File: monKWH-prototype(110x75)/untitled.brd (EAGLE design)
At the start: 69.4 x 109.6 mm, 26 parts, among them J1 U.FL-R-SMT(01), X1 MSTBA2

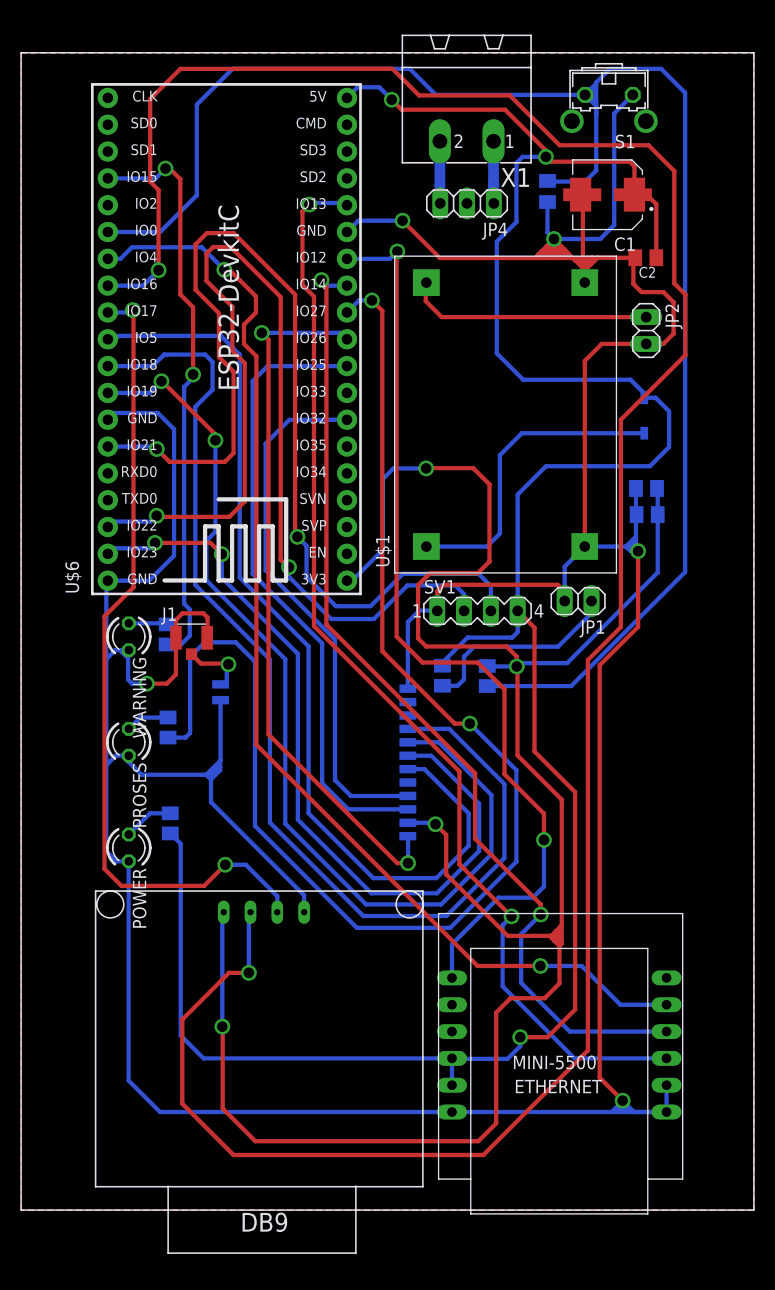
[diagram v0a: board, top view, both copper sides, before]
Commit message: perubahan mikro dan penambahan Jack-DC
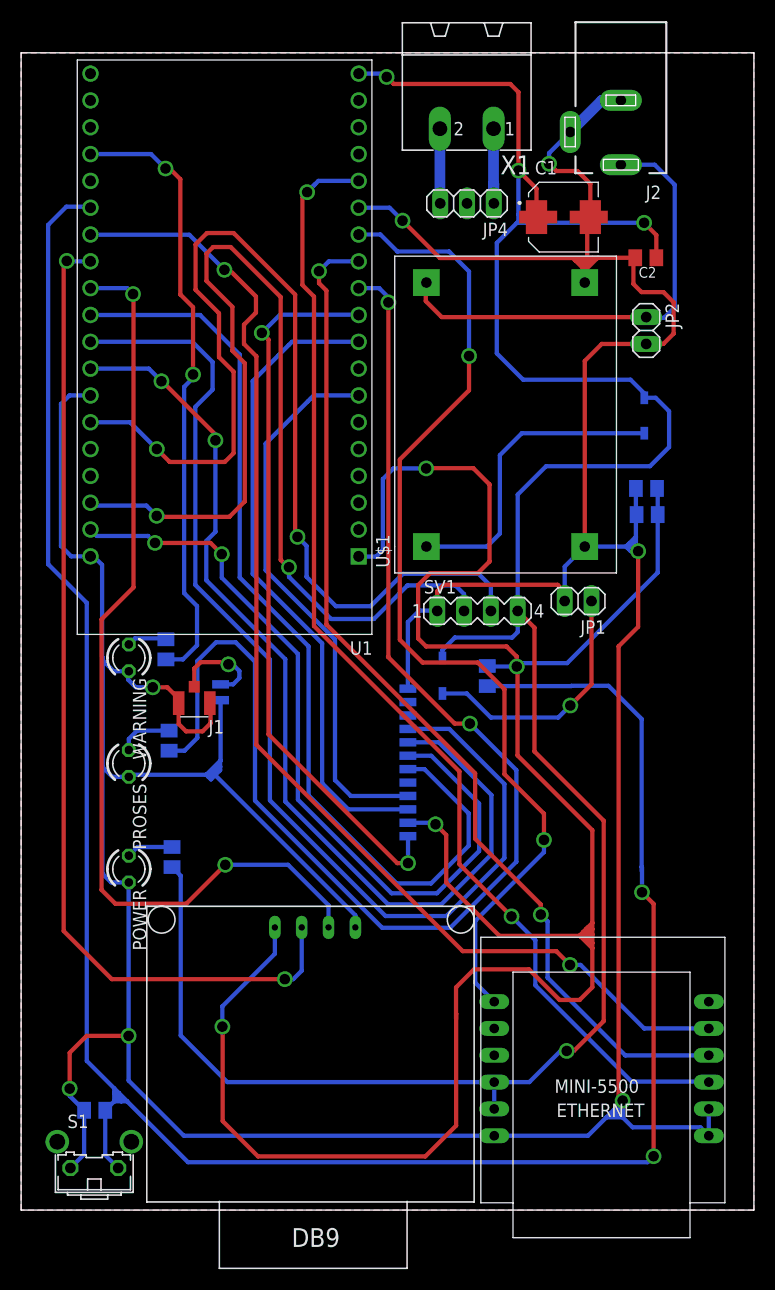
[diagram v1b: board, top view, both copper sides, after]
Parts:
- removed U$6: ESP32DEVKITC, ESP32-DEVKITC:ESP32-DEVKITC
- added J2: DCJ0202, con-jack:DCJ0202
- added U1: ESP32-DEVKITC-32D, ESP32-DEVKITC-32D:MODULE_ESP32-DEVKITC-32D
- R2: device adafruit:M0805 -> 1N5819HW-7:SOD3715X145N
- moved S1 110.5 mm to (3.73, 3.93), turned to 0 degrees
- moved C3 97.0 mm to (3.77, 8.15), turned to 0 degrees
- moved J1 6.19 mm to (13.2, 46.7), turned to 180 degrees
- moved U$5 5.06 mm to (39.7, 27.5)
- moved C1 4.69 mm to (48.2, 92.7), turned to 0 degrees
- moved U$3 4.59 mm to (63.5, -0.61)
- moved R1 3.19 mm to (11.1, 32.1)
- moved POWER 2.00 mm to (7.00, 31.0)
- moved PROSES 2.00 mm to (7.00, 41.0)
- moved WARNING 2.00 mm to (7.00, 51.0)
- moved R16 1.41 mm to (10.5, 51.8)
- moved R3 1.25 mm to (10.8, 43.2)
- moved X1 1.19 mm to (39.0, 106.2)
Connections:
- removed net EN: U$6.2
- removed net RST_LAN1: U$6.8
- net 3V3: now also U1.1; no longer U$6.1
- net GND: now also J2.2, J2.3, U1.14, U1.20, U1.26; no longer U$6.14, U$6.32, U$6.38
- net LED_PROSES: now also U1.11; no longer U$6.11
- net LED_WARNING: now also U1.35; no longer U$6.23
- net LORA_DI0: now also U1.9; no longer U$6.9
- net LORA_DI1: now also U1.7; no longer U$6.7
- net MISO_HSPI: now also U1.13; no longer U$6.13
- net MISO_VSPI: now also U1.21; no longer U$6.37
- net MOSI_HSPI: now also U1.15; no longer U$6.15
- net MOSI_VSPI: now also U1.27; no longer U$6.31
- net N$4: now also J2.1
- net N$7: now also R2.A; no longer R2.2
- net OUT+: now also R2.C, U1.19; no longer R2.1, U$6.19
- net RST: now also U1.33; no longer U$6.25
- net RST_LORA: now also U1.10; no longer U$6.10
- net RX_DB9: now also U1.31; no longer U$6.27
- net SCK_HSPI: now also U1.12; no longer U$6.12
- net SCK_VSPI: now also U1.28; no longer U$6.30
- net SCL: now also U1.22; no longer U$6.36
- net SDA: now also U1.25; no longer U$6.33
- net SS_LAN_CONV: now also U1.32; no longer U$6.26
- net SS_LORA: now also U1.29; no longer U$6.29
- net TX_DB9: now also U1.30; no longer U$6.28
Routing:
- net RX_DB9: track 230.8 -> 94.7 mm
- net RST: track 156.7 -> 213.2 mm, vias 0 -> 2
- net N$4: track 23.3 -> 43.9 mm
- net 3V3: track 203.9 -> 217.2 mm
- net TX_DB9: track 77.2 -> 89.2 mm
- net MISO_HSPI: track 88.2 -> 95.9 mm
- net GND: track 423.1 -> 415.7 mm, vias 5 -> 7
- net SS_LAN_CONV: track 108.9 -> 115.5 mm
- net MOSI_HSPI: track 104.9 -> 111.1 mm
- net N$7: track 19.5 -> 24.2 mm, vias 0 -> 1
- net LED_WARNING: track 54.5 -> 58.5 mm
- net SCK_HSPI: track 94.4 -> 98.3 mm
- net OUT+: track 226.0 -> 229.5 mm, vias 3 -> 4
- net ANT: track 6.39 -> 9.29 mm
- net SDA: track 96.3 -> 98.9 mm
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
